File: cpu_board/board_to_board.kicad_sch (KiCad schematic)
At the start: 2 parts

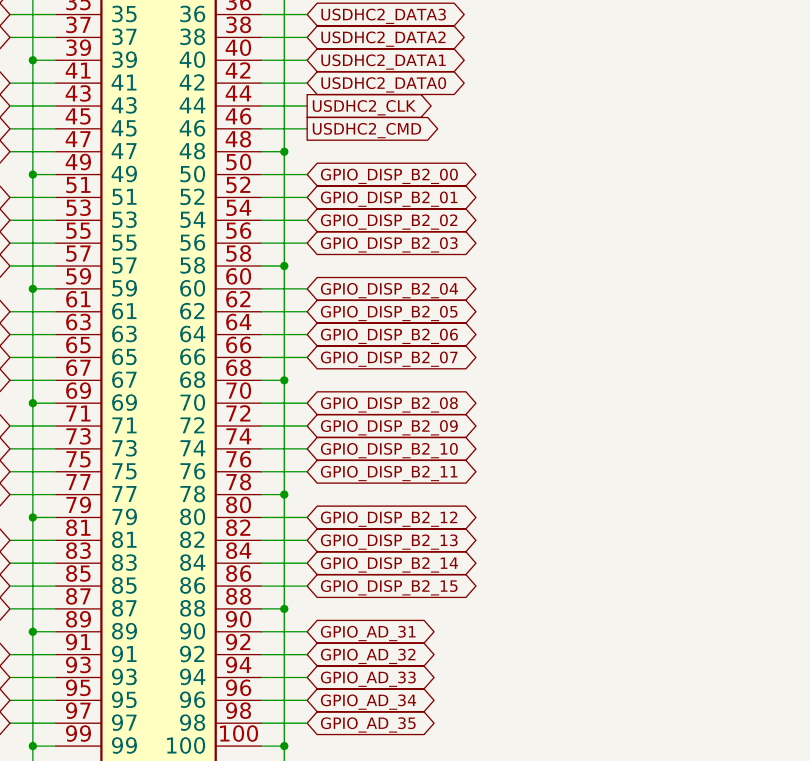
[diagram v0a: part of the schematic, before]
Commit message: grounded
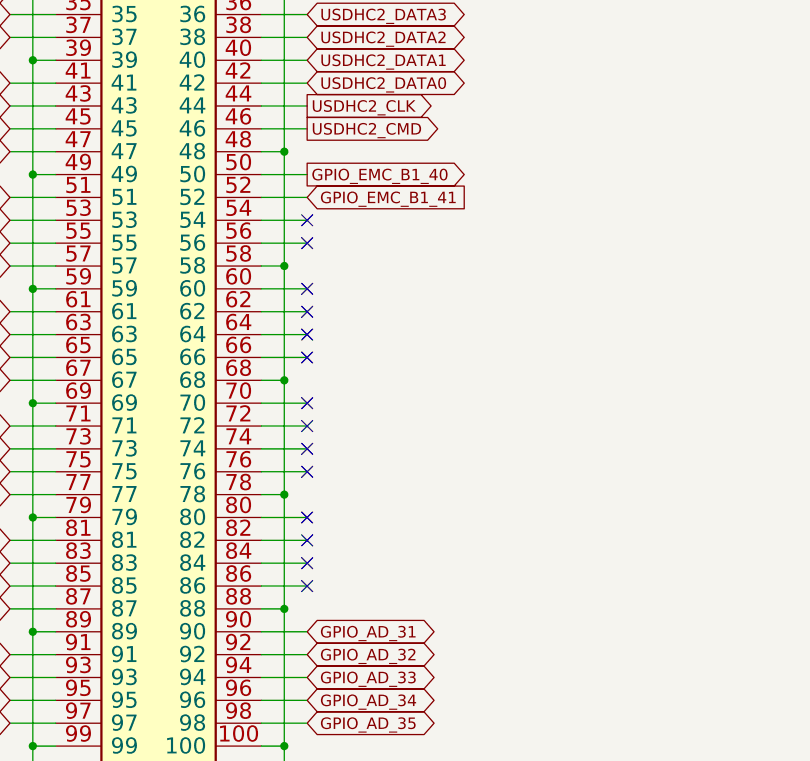
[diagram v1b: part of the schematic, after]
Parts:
- J? (x2): footprint adcs:HIROSE_DF40C-100DP-0.4V(51) -> adcs:DF40C100DP04V51
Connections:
- net GPIO_DISP_B2_00: no longer J?.50
- net GPIO_DISP_B2_01: no longer J?.52
- net GPIO_DISP_B2_02: no longer J?.54
- net GPIO_DISP_B2_03: no longer J?.56
- net GPIO_DISP_B2_04: no longer J?.60
- net GPIO_DISP_B2_05: no longer J?.62
- net GPIO_DISP_B2_06: no longer J?.64
- net GPIO_DISP_B2_07: no longer J?.66
- net GPIO_DISP_B2_08: no longer J?.70
- net GPIO_DISP_B2_09: no longer J?.72
- net GPIO_DISP_B2_10: no longer J?.74
- net GPIO_DISP_B2_11: no longer J?.76
- net GPIO_DISP_B2_12: no longer J?.80
- net GPIO_DISP_B2_13: no longer J?.82
- net GPIO_DISP_B2_14: no longer J?.84
- net GPIO_DISP_B2_15: no longer J?.86
- new net GPIO_EMC_B1_40: J?.50
- new net GPIO_EMC_B1_41: J?.52
- no-connect marks 0 -> 14
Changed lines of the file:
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@@
   (junction (at 99.06 107.95) (diameter 0) (color 0 0 0 0)
   )
+  (no_connect (at 129.54 151.13))
+  (no_connect (at 129.54 166.37))
+  (no_connect (at 129.54 171.45))
+  (no_connect (at 129.54 184.15))
+  (no_connect (at 129.54 186.69))
+  (no_connect (at 129.54 176.53))
+  (no_connect (at 129.54 158.75))
+  (no_connect (at 129.54 153.67))
+  (no_connect (at 129.54 173.99))
+  (no_connect (at 129.54 191.77))
+  (no_connect (at 129.54 189.23))
+  (no_connect (at 129.54 163.83))
+  (no_connect (at 129.54 179.07))
+  (no_connect (at 129.54 161.29))
   (wire (pts (xy 307.975 186.055) (xy 310.515 186.055))
     (stroke (width 0) (type default))
@@
     )
   )
-  (global_label "GPIO_DISP_B2_02" (shape bidirectional) (at 129.54 151.13 0) (fields_autoplaced)
-    (effects (font (size 1.27 1.27)) (justify left))
-    (property "Intersheetrefs" "${INTERSHEET_REFS}" (at 147.3043 151.13 0)
-      (effects (font (size 1.27 1.27)) (justify left) hide)
-    )
-  )
   (global_label "GPIO_AD_10" (shape bidirectional) (at 96.52 148.59 180) (fields_autoplaced)
     (effects (font (size 1.27 1.27)) (justify right))
@@
     )
   )
-  (global_label "GPIO_DISP_B2_12" (shape bidirectional) (at 129.54 184.15 0) (fields_autoplaced)
-    (effects (font (size 1.27 1.27)) (justify left))
-    (property "Intersheetrefs" "${INTERSHEET_REFS}" (at 147.3043 184.15 0)
-      (effects (font (size 1.27 1.27)) (justify left) hide)
-    )
-  )
-  (global_label "GPIO_DISP_B2_15" (shape bidirectional) (at 129.54 191.77 0) (fields_autoplaced)
-    (effects (font (size 1.27 1.27)) (justify left))
-    (property "Intersheetrefs" "${INTERSHEET_REFS}" (at 147.3043 191.77 0)
-      (effects (font (size 1.27 1.27)) (justify left) hide)
-    )
-  )
   (global_label "GPIO_SD_B1_03" (shape bidirectional) (at 129.54 118.11 0) (fields_autoplaced)
     (effects (font (size 1.27 1.27)) (justify left))
@@
     )
   )
+  (global_label "GPIO_EMC_B1_41" (shape input) (at 129.54 148.59 0)
+    (effects (font (size 1.27 1.27)) (justify left))
+    (property "Intersheetrefs" "${INTERSHEET_REFS}" (at 129.54 148.59 0)
+      (effects (font (size 1.27 1.27)) hide)
+    )
+  )
   (global_label "GPIO_EMC_B2_08" (shape bidirectional) (at 278.765 155.575 180)
     (effects (font (size 1.27 1.27)) (justify right))
@@
     )
   )
-  (global_label "GPIO_DISP_B2_00" (shape bidirectional) (at 129.54 146.05 0) (fields_autoplaced)
-    (effects (font (size 1.27 1.27)) (justify left))
-    (property "Intersheetrefs" "${INTERSHEET_REFS}" (at 148.0448 146.05 0)
-      (effects (font (size 1.27 1.27)) (justify left) hide)
-    )
-  )
   (global_label "GPIO_AD_28" (shape bidirectional) (at 96.52 201.93 180) (fields_autoplaced)
     (effects (font (size 1.27 1.27)) (justify right))
@@
     )
   )
-  (global_label "GPIO_DISP_B2_05" (shape bidirectional) (at 129.54 161.29 0) (fields_autoplaced)
-    (effects (font (size 1.27 1.27)) (justify left))
-    (property "Intersheetrefs" "${INTERSHEET_REFS}" (at 147.3043 161.29 0)
-      (effects (font (size 1.27 1.27)) (justify left) hide)
-    )
-  )
   (global_label "GPIO_AD_15" (shape bidirectional) (at 96.52 163.83 180) (fields_autoplaced)
     (effects (font (size 1.27 1.27)) (justify right))
@@
     )
   )
-  (global_label "GPIO_DISP_B2_03" (shape bidirectional) (at 129.54 153.67 0) (fields_autoplaced)
-    (effects (font (size 1.27 1.27)) (justify left))
-    (property "Intersheetrefs" "${INTERSHEET_REFS}" (at 147.3043 153.67 0)
-      (effects (font (size 1.27 1.27)) (justify left) hide)
-    )
-  )
   (global_label "MIPI_CSI_D0_P" (shape input) (at 313.055 188.595 0) (fields_autoplaced)
     (effects (font (size 1.27 1.27)) (justify left))
@@
     )
   )
-  (global_label "GPIO_DISP_B2_09" (shape bidirectional) (at 129.54 173.99 0) (fields_autoplaced)
-    (effects (font (size 1.27 1.27)) (justify left))
-    (property "Intersheetrefs" "${INTERSHEET_REFS}" (at 147.3043 173.99 0)
-      (effects (font (size 1.27 1.27)) (justify left) hide)
-    )
-  )
-  (global_label "GPIO_DISP_B2_08" (shape bidirectional) (at 129.54 171.45 0) (fields_autoplaced)
-    (effects (font (size 1.27 1.27)) (justify left))
-    (property "Intersheetrefs" "${INTERSHEET_REFS}" (at 147.3043 171.45 0)
-      (effects (font (size 1.27 1.27)) (justify left) hide)
-    )
-  )
   (global_label "GPIO_AD_01" (shape bidirectional) (at 96.52 118.11 180) (fields_autoplaced)
     (effects (font (size 1.27 1.27)) (justify right))
@@
     )
   )
-  (global_label "GPIO_DISP_B2_13" (shape bidirectional) (at 129.54 186.69 0) (fields_autoplaced)
-    (effects (font (size 1.27 1.27)) (justify left))
-    (property "Intersheetrefs" "${INTERSHEET_REFS}" (at 147.3043 186.69 0)
-      (effects (font (size 1.27 1.27)) (justify left) hide)
-    )
-  )
-  (global_label "GPIO_DISP_B2_11" (shape bidirectional) (at 129.54 179.07 0) (fields_autoplaced)
-    (effects (font (size 1.27 1.27)) (justify left))
-    (property "Intersheetrefs" "${INTERSHEET_REFS}" (at 147.3043 179.07 0)
-      (effects (font (size 1.27 1.27)) (justify left) hide)
-    )
-  )
   (global_label "USDHC2_DATA2" (shape bidirectional) (at 129.54 130.81 0) (fields_autoplaced)
     (effects (font (size 1.27 1.27)) (justify left))
@@
     )
   )
-  (global_label "GPIO_DISP_B2_06" (shape bidirectional) (at 129.54 163.83 0) (fields_autoplaced)
-    (effects (font (size 1.27 1.27)) (justify left))
-    (property "Intersheetrefs" "${INTERSHEET_REFS}" (at 147.3043 163.83 0)
-      (effects (font (size 1.27 1.27)) (justify left) hide)
+  (global_label "GPIO_EMC_B1_40" (shape output) (at 129.54 146.05 0)
+    (effects (font (size 1.27 1.27)) (justify left))
+    (property "Intersheetrefs" "${INTERSHEET_REFS}" (at 129.54 146.05 0)
+      (effects (font (size 1.27 1.27)) hide)
     )
   )
@@
     )
   )
-  (global_label "GPIO_DISP_B2_10" (shape bidirectional) (at 129.54 176.53 0) (fields_autoplaced)
-    (effects (font (size 1.27 1.27)) (justify left))
-    (property "Intersheetrefs" "${INTERSHEET_REFS}" (at 147.3043 176.53 0)
-      (effects (font (size 1.27 1.27)) (justify left) hide)
-    )
-  )
   (global_label "GPIO_DISP_B2_11" (shape bidirectional) (at 313.055 173.355 0) (fields_autoplaced)
     (effects (font (size 1.27 1.27)) (justify left))
@@
     )
   )
-  (global_label "GPIO_DISP_B2_07" (shape bidirectional) (at 129.54 166.37 0) (fields_autoplaced)
-    (effects (font (size 1.27 1.27)) (justify left))
-    (property "Intersheetrefs" "${INTERSHEET_REFS}" (at 147.3043 166.37 0)
-      (effects (font (size 1.27 1.27)) (justify left) hide)
-    )
-  )
   (global_label "GPIO_LPSR_07" (shape bidirectional) (at 96.52 105.41 180) (fields_autoplaced)
     (effects (font (size 1.27 1.27)) (justify right))
@@
     )
   )
-  (global_label "GPIO_DISP_B2_01" (shape bidirectional) (at 129.54 148.59 0) (fields_autoplaced)
-    (effects (font (size 1.27 1.27)) (justify left))
-    (property "Intersheetrefs" "${INTERSHEET_REFS}" (at 147.3043 148.59 0)
-      (effects (font (size 1.27 1.27)) (justify left) hide)
-    )
-  )
   (global_label "GPIO_DISP_B1_05" (shape bidirectional) (at 313.055 117.475 0) (fields_autoplaced)
     (effects (font (size 1.27 1.27)) (justify left))
@@
     )
   )
-  (global_label "GPIO_DISP_B2_14" (shape bidirectional) (at 129.54 189.23 0) (fields_autoplaced)
-    (effects (font (size 1.27 1.27)) (justify left))
-    (property "Intersheetrefs" "${INTERSHEET_REFS}" (at 147.3043 189.23 0)
-      (effects (font (size 1.27 1.27)) (justify left) hide)
-    )
-  )
   (global_label "GPIO_EMC_B2_00" (shape bidirectional) (at 278.765 132.715 180)
     (effects (font (size 1.27 1.27)) (justify right))
@@
     (effects (font (size 1.27 1.27)) (justify left))
     (property "Intersheetrefs" "${INTERSHEET_REFS}" (at 148.3926 120.65 0)
-      (effects (font (size 1.27 1.27)) (justify left) hide)
-    )
-  )
-  (global_label "GPIO_DISP_B2_04" (shape bidirectional) (at 129.54 158.75 0) (fields_autoplaced)
-    (effects (font (size 1.27 1.27)) (justify left))
-    (property "Intersheetrefs" "${INTERSHEET_REFS}" (at 147.3043 158.75 0)
       (effects (font (size 1.27 1.27)) (justify left) hide)
     )
@@
       (effects (font (size 1.27 1.27)) hide)
     )
-    (property "Footprint" "adcs:HIROSE_DF40C-100DP-0.4V(51)" (at 106.68 80.01 0)
+    (property "Footprint" "adcs:DF40C100DP04V51" (at 106.68 80.01 0)
       (effects (font (size 1.27 1.27)) hide)
     )
@@
     (property "Footprint (for JLCPCB)" "" (at 106.68 80.01 0)
       (effects (font (size 1.27 1.27)) hide)
+    )
+    (property "DigiKey Part Number" "" (at 106.68 80.01 0)
+      (effects (font (size 1.27 1.27)) hide)
+    )
+    (property "Tolerance" "" (at 106.68 80.01 0)
+      (effects (font (size 1.27 1.27)))
+    )
+    (property "Power Rating" "" (at 106.68 80.01 0)
+      (effects (font (size 1.27 1.27)))
     )
     (pin "1")
@@
       (effects (font (size 1.27 1.27)) hide)
     )
-    (property "Footprint" "adcs:HIROSE_DF40C-100DP-0.4V(51)" (at 290.195 76.835 0)
+    (property "Footprint" "adcs:DF40C100DP04V51" (at 290.195 76.835 0)
       (effects (font (size 1.27 1.27)) hide)
     )
@@
       (effects (font (size 1.27 1.27)) hide)
     )
+    (property "DigiKey Part Number" "" (at 290.195 76.835 0)
+      (effects (font (size 1.27 1.27)) hide)
+    )
+    (property "Tolerance" "" (at 290.195 76.835 0)
+      (effects (font (size 1.27 1.27)))
+    )
+    (property "Power Rating" "" (at 290.195 76.835 0)
+      (effects (font (size 1.27 1.27)))
+    )
     (pin "1")
